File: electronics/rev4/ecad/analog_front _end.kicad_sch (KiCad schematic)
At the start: 24 parts, among them J3 Red Banana Plug, J4 Black Banana Plug, Q25 2N7002, SW3 GF-161-0005, U10 MCP3561, U3 OPA4388IDR

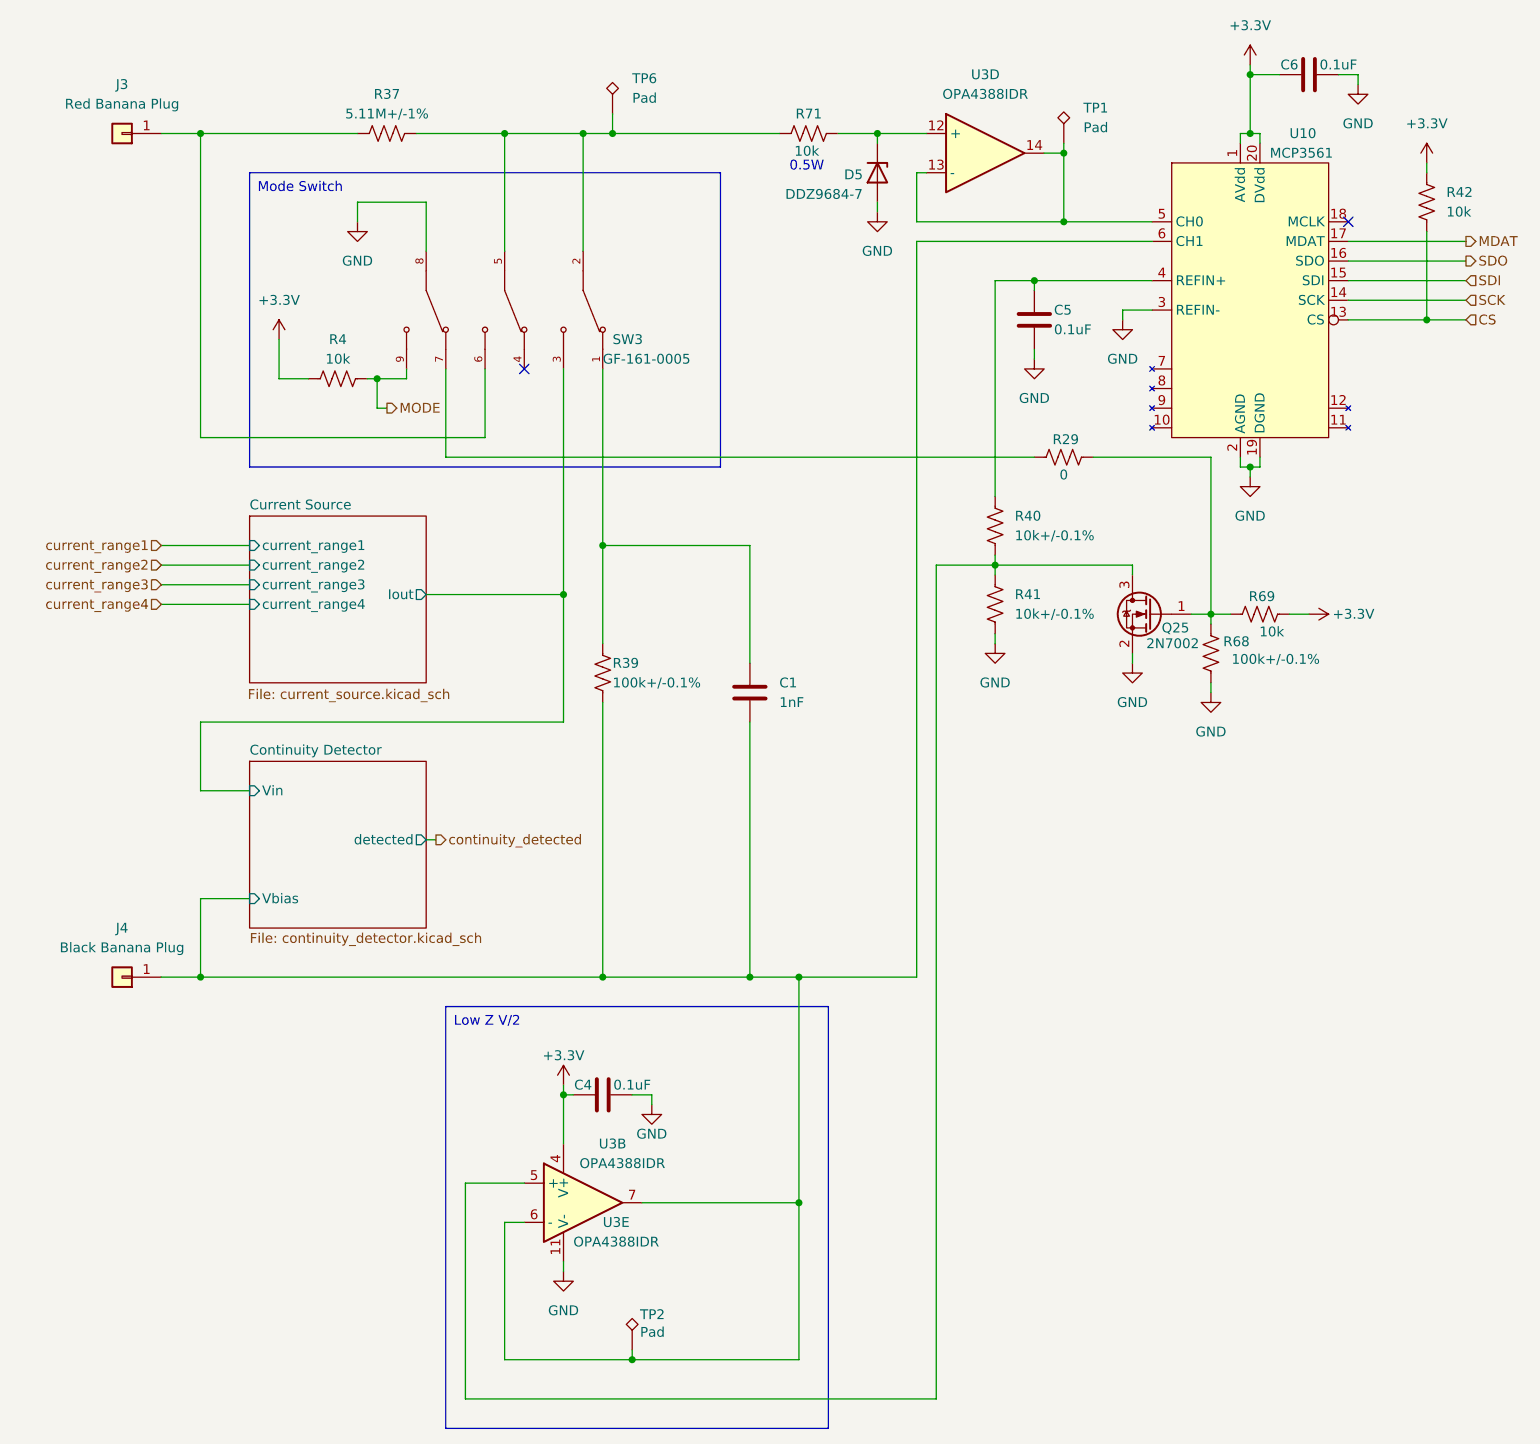
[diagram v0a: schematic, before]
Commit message: started rev4
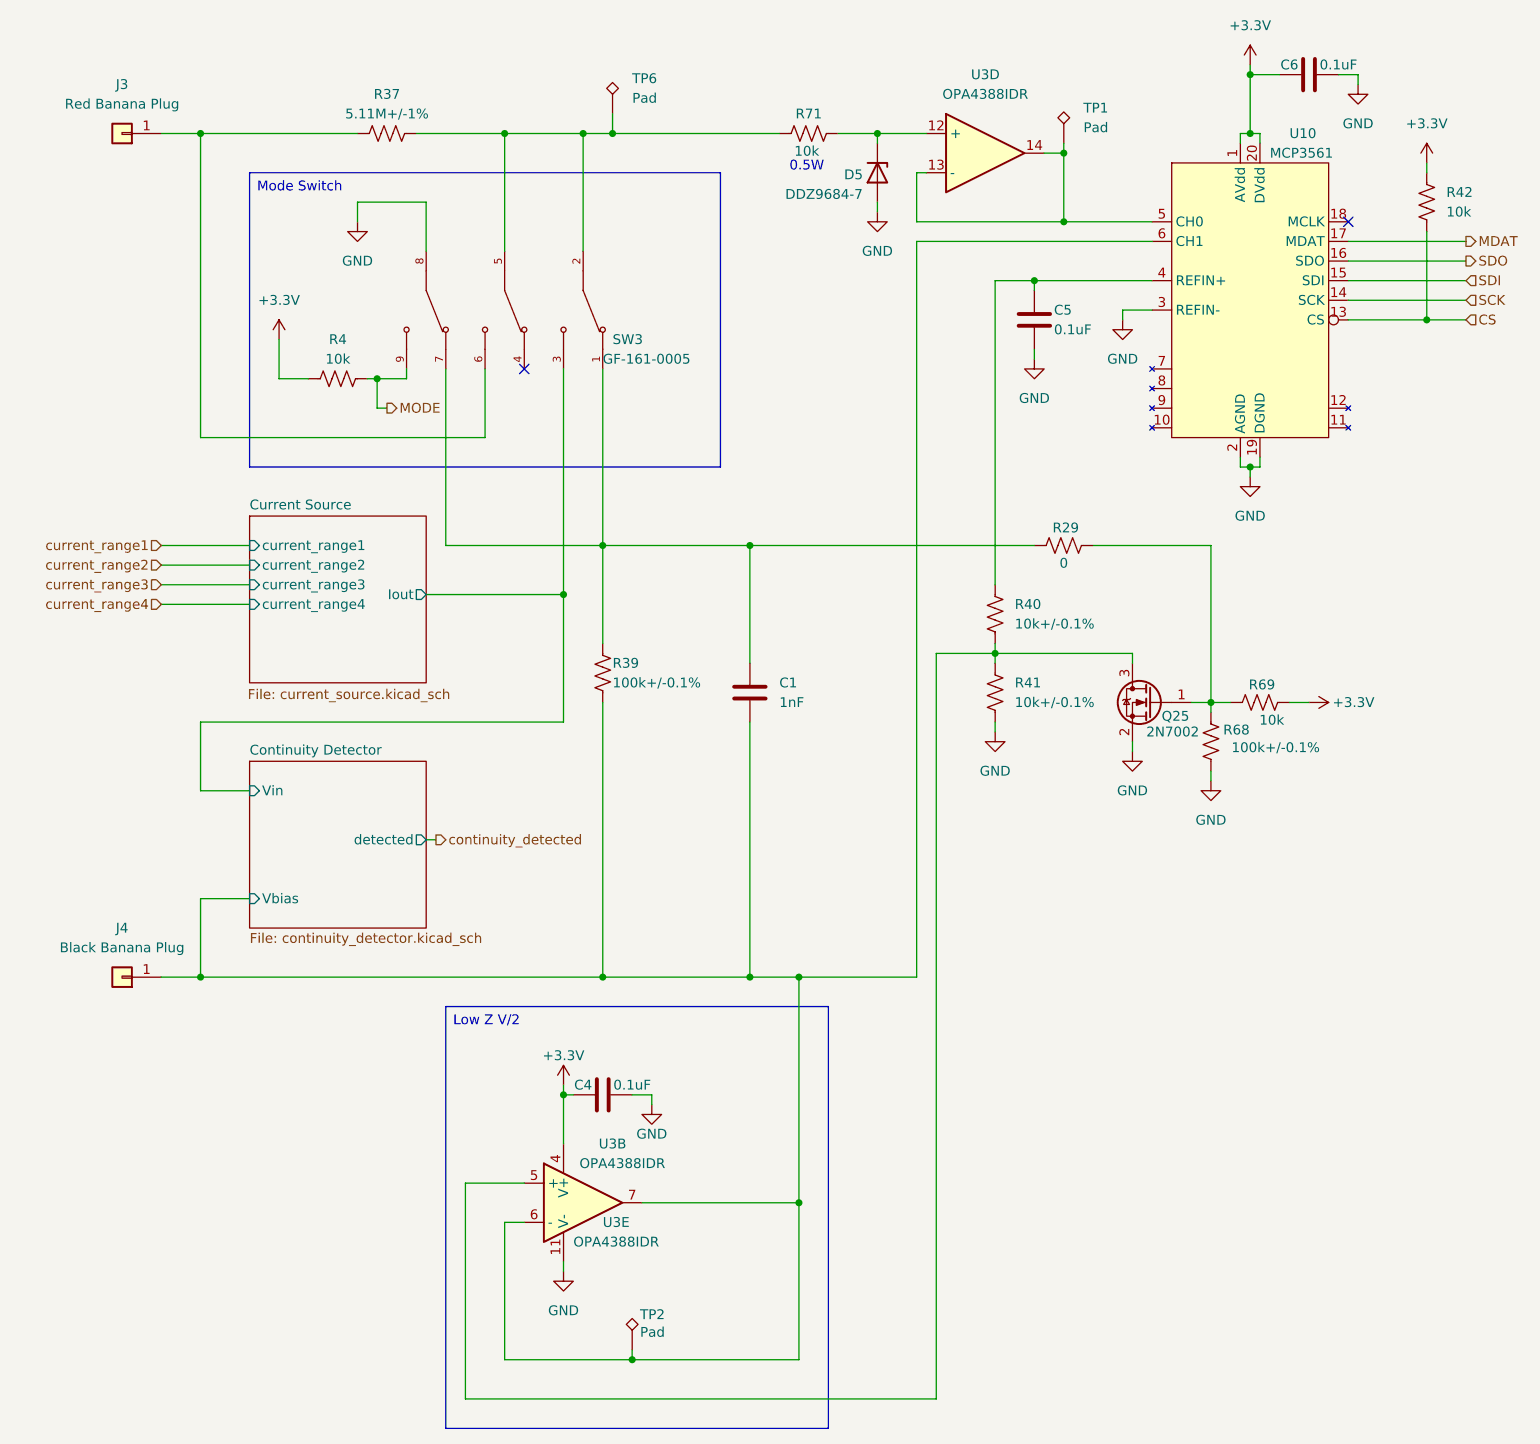
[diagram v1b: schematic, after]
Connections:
- net at C1.1, R39.1, SW3.1: now also R29.1, SW3.7
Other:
- moved on the sheet: Q25, R29, R40, R41, R68, R69
